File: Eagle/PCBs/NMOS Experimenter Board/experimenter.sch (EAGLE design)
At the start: 1211 parts, among them Q10 2N7002, Q11 2N7002, Q12 2N7002, Q13 2N7002, Q14 2N7002, Q15 2N7002, Q16 2N7002, Q17 2N7002, Q18 2N7002, Q19 2N7002, Q2 2N7002, Q20 2N7002, Q21 2N7002, Q22 2N7002, Q23 2N7002, Q24 2N7002, Q25 2N7002, Q26 2N7002, Q27 2N7002, Q28 2N7002, Q29 2N7002, Q3 2N7002, Q30 2N7002, Q31 2N7002, Q32 2N7002, Q33 2N7002, Q34 2N7002, Q35 2N7002, Q36 2N7002, Q37 2N7002, Q38 2N7002, Q39 2N7002, Q4 2N7002, Q40 2N7002, Q41 2N7002, Q42 2N7002, Q43 2N7002, Q44 2N7002, Q45 2N7002, Q46 2N7002, Q47 2N7002, Q48 2N7002, Q49 2N7002, Q5 2N7002, Q50 2N7002, Q51 2N7002, Q52 2N7002, Q53 2N7002, Q54 2N7002, Q55 2N7002, Q56 2N7002, Q57 2N7002, Q58 2N7002, Q59 2N7002, Q6 2N7002, Q60 2N7002, Q61 2N7002, Q62 2N7002, Q63 2N7002, Q64 2N7002, Q65 2N7002, Q66 2N7002, Q67 2N7002, Q68 2N7002, Q69 2N7002, Q7 2N7002, Q70 2N7002, Q71 2N7002, Q72 2N7002, Q73 2N7002, Q8 2N7002, Q9 2N7002, U1 74HC14PW, U2 74HC14PW

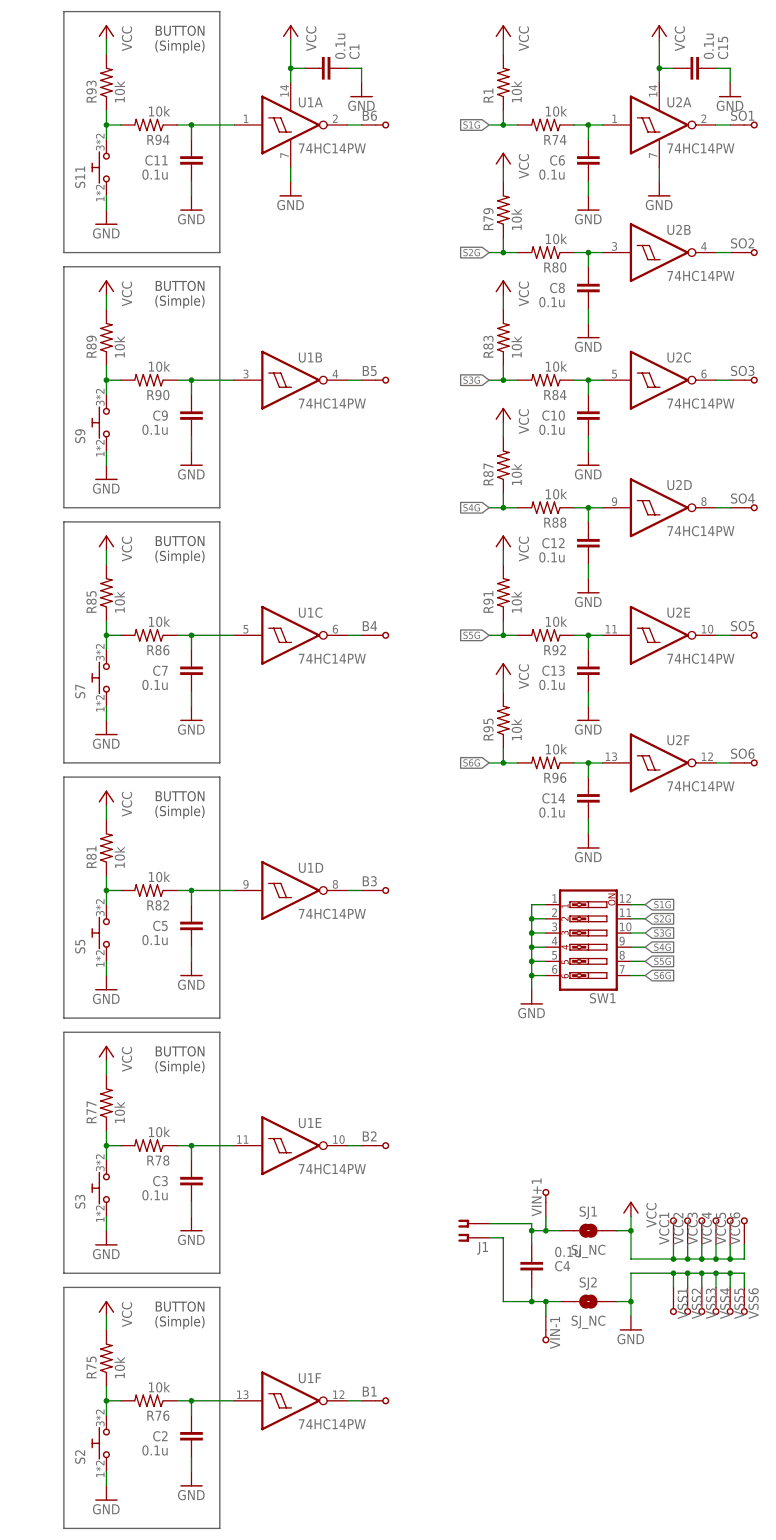
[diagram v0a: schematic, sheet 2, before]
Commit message: Start rework on experimenter
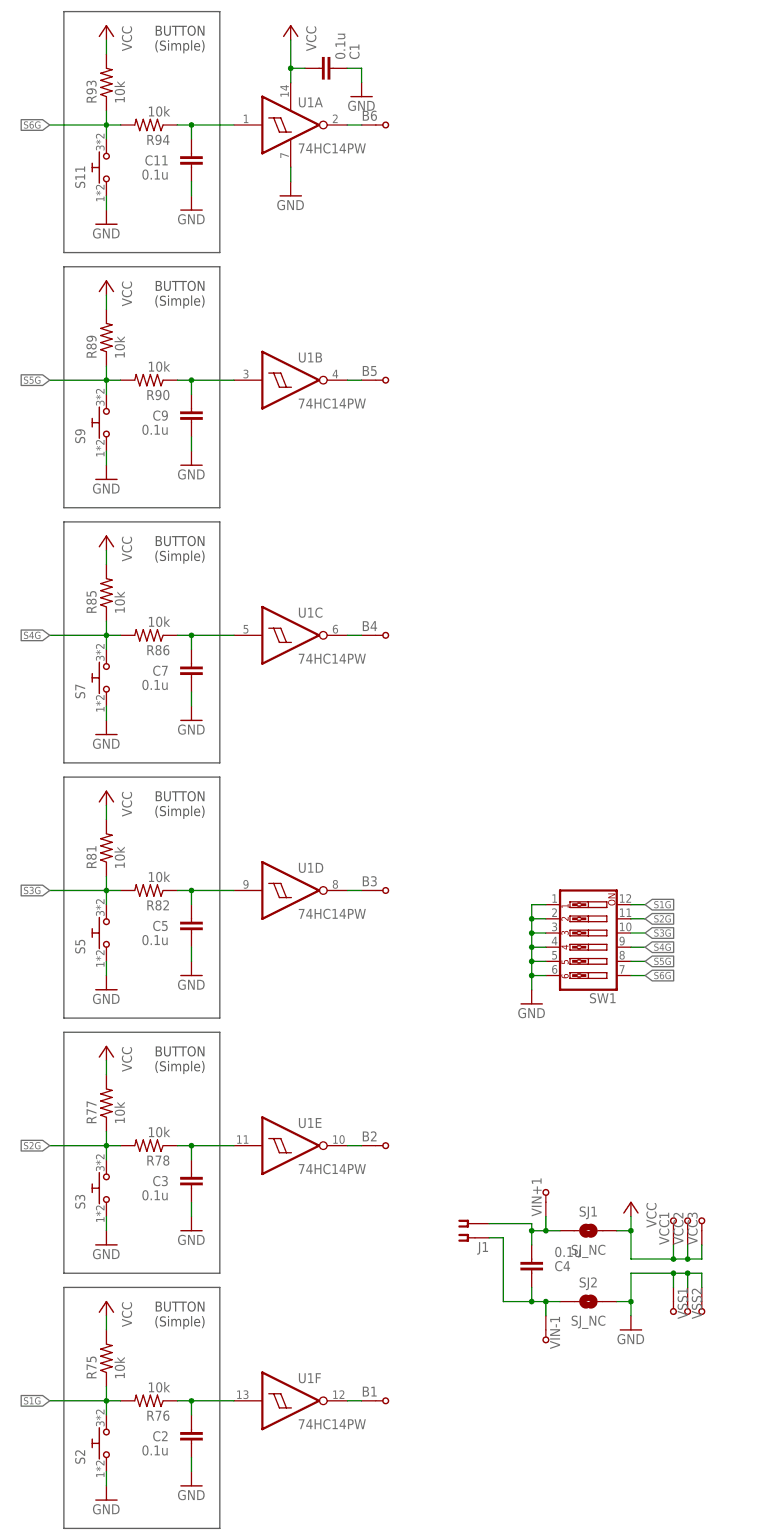
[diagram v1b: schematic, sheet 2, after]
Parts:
- removed C10, C12, C13, C14, C15, C6, C8: 0.1u, ellajameson-core:CAP0603
- removed D10, D11, D12, D13, D14, D15, D16, D17, D18, D19, D2, D20, D21, D22, D23, D24, D25, D26, D27, D28, D29, D3, D30, D31, D32, D33, D34, D35, D36, D37, D38, D39, D4, D40, D41, D42, D43, D44, D45, D46, D47, D48, D49, D5, D50, D51, D52, D53, D54, D55, D56, D57, D58, D59, D6, D60, D61, D62, D63, D64, D65, D66, D67, D68, D69, D7, D70, D71, D72, D73, D8, D9: (no value), ellajameson-core:LED0603
- removed DRAINA10, DRAINA11, DRAINA12, DRAINA13, DRAINA14, DRAINA15, DRAINA16, DRAINA17, DRAINA18, DRAINA19, DRAINA2, DRAINA20, DRAINA21, DRAINA22, DRAINA23, DRAINA24, DRAINA25, DRAINA26, DRAINA27, DRAINA28, DRAINA29, DRAINA3, DRAINA30, DRAINA31, DRAINA32, DRAINA33, DRAINA34, DRAINA35, DRAINA36, DRAINA37, DRAINA38, DRAINA39, DRAINA4, DRAINA40, DRAINA41, DRAINA42, DRAINA43, DRAINA44, DRAINA45, DRAINA46, DRAINA47, DRAINA48, DRAINA49, DRAINA5, DRAINA50, DRAINA51, DRAINA52, DRAINA53, DRAINA54, DRAINA55, DRAINA56, DRAINA57, DRAINA58, DRAINA59, DRAINA6, DRAINA60, DRAINA61, DRAINA62, DRAINA63, DRAINA64, DRAINA65, DRAINA66, DRAINA67, DRAINA68, DRAINA69, DRAINA7, DRAINA70, DRAINA71, DRAINA72, DRAINA73, DRAINA8, DRAINA9, DRAINB10, DRAINB11, DRAINB12, DRAINB13, DRAINB14, DRAINB15, DRAINB16, DRAINB17, DRAINB18, DRAINB19, DRAINB2, DRAINB20, DRAINB21, DRAINB22, DRAINB23, DRAINB24, DRAINB25, DRAINB26, DRAINB27, DRAINB28, DRAINB29, DRAINB3, DRAINB30, DRAINB31, DRAINB32, DRAINB33, DRAINB34, DRAINB35, DRAINB36, DRAINB37, DRAINB38, DRAINB39, DRAINB4, DRAINB40, DRAINB41, DRAINB42, DRAINB43, DRAINB44, DRAINB45, DRAINB46, DRAINB47, DRAINB48, DRAINB49, DRAINB5, DRAINB50, DRAINB51, DRAINB52, DRAINB53, DRAINB54, DRAINB55, DRAINB56, DRAINB57, DRAINB58, DRAINB59, DRAINB6, DRAINB60, DRAINB61, DRAINB62, DRAINB63, DRAINB64, DRAINB65, DRAINB66, DRAINB67, DRAINB68, DRAINB69, DRAINB7, DRAINB70, DRAINB71, DRAINB72, DRAINB73, DRAINB8, DRAINB9, DRAINC10, DRAINC11, DRAINC12, DRAINC13, DRAINC14, DRAINC15, DRAINC16, DRAINC17, DRAINC18, DRAINC19, DRAINC2, DRAINC20, DRAINC21, DRAINC22, DRAINC23, DRAINC24, DRAINC25, DRAINC26, DRAINC27, DRAINC28, DRAINC29, DRAINC3, DRAINC30, DRAINC31, DRAINC32, DRAINC33, DRAINC34, DRAINC35, DRAINC36, DRAINC37, DRAINC38, DRAINC39, DRAINC4, DRAINC40, DRAINC41, DRAINC42, DRAINC43, DRAINC44, DRAINC45, DRAINC46, DRAINC47, DRAINC48, DRAINC49, DRAINC5, DRAINC50, DRAINC51, DRAINC52, DRAINC53, DRAINC54, DRAINC55, DRAINC56, DRAINC57, DRAINC58, DRAINC59, DRAINC6, DRAINC60, DRAINC61, DRAINC62, DRAINC63, DRAINC64, DRAINC65, DRAINC66, DRAINC67, DRAINC68, DRAINC69, DRAINC7, DRAINC70, DRAINC71, DRAINC72, DRAINC73, DRAINC8, DRAINC9, DRAIND10, DRAIND11, DRAIND12, DRAIND13, DRAIND14, DRAIND15, DRAIND16, DRAIND17, DRAIND18, DRAIND19, DRAIND2, DRAIND20, DRAIND21, DRAIND22, DRAIND23, DRAIND24, DRAIND25, DRAIND26, DRAIND27, DRAIND28, DRAIND29, DRAIND3, DRAIND30, DRAIND31, DRAIND32, DRAIND33, DRAIND34, DRAIND35, DRAIND36, DRAIND37, DRAIND38, DRAIND39, DRAIND4, DRAIND40, DRAIND41, DRAIND42, DRAIND43, DRAIND44, DRAIND45, DRAIND46, DRAIND47, DRAIND48, DRAIND49, DRAIND5, DRAIND50, DRAIND51, DRAIND52, DRAIND53, DRAIND54, DRAIND55, DRAIND56, DRAIND57, DRAIND58, DRAIND59, DRAIND6, DRAIND60, DRAIND61, DRAIND62, DRAIND63, DRAIND64, DRAIND65, DRAIND66, DRAIND67, DRAIND68, DRAIND69, DRAIND7, DRAIND70, DRAIND71, DRAIND72, DRAIND73, DRAIND8, DRAIND9, GATE10, GATE11, GATE12, GATE13, GATE14, GATE15, GATE16, GATE17, GATE18, GATE19, GATE2, GATE20, GATE21, GATE22, GATE23, GATE24, GATE25, GATE26, GATE27, GATE28, GATE29, GATE3, GATE30, GATE31, GATE32, GATE33, GATE34, GATE35, GATE36, GATE37, GATE38, GATE39, GATE4, GATE40, GATE41, GATE42, GATE43, GATE44, GATE45, GATE46, GATE47, GATE48, GATE49, GATE5, GATE50, GATE51, GATE52, GATE53, GATE54, GATE55, GATE56, GATE57, GATE58, GATE59, GATE6, GATE60, GATE61, GATE62, GATE63, GATE64, GATE65, GATE66, GATE67, GATE68, GATE69, GATE7, GATE70, GATE71, GATE72, GATE73, GATE8, GATE9, SO1, SO2, SO3, SO4, SO5, SO6, SOURCEA10, SOURCEA11, SOURCEA12, SOURCEA13, SOURCEA14, SOURCEA15, SOURCEA16, SOURCEA17, SOURCEA18, SOURCEA19, SOURCEA2, SOURCEA20, SOURCEA21, SOURCEA22, SOURCEA23, SOURCEA24, SOURCEA25, SOURCEA26, SOURCEA27, SOURCEA28, SOURCEA29, SOURCEA3, SOURCEA30, SOURCEA31, SOURCEA32, SOURCEA33, SOURCEA34, SOURCEA35, SOURCEA36, SOURCEA37, SOURCEA38, SOURCEA39, SOURCEA4, SOURCEA40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: TPWIRE, ellajameson-core:TPWIRE
- removed JD10, JD11, JD12, JD13, JD14, JD17, JD18, JD19, JD2, JD20, JD21, JD22, JD23, JD24, JD25, JD26, JD27, JD28, JD29, JD3, JD30, JD31, JD32, JD33, JD34, JD35, JD36, JD37, JD38, JD39, JD4, JD40, JD41, JD42, JD43, JD44, JD45, JD46, JD47, JD48, JD49, JD5, JD50, JD51, JD52, JD53, JD54, JD55, JD56, JD57, JD58, JD59, JD6, JD60, JD61, JD62, JD63, JD64, JD65, JD66, JD68, JD7, JD70, JD72, JD8, JD9, JN10, JN11, JN12, JN13, JN14, JN15, JN16, JN17, JN18, JN19, JN2, JN20, JN21, JN22, JN23, JN24, JN25, JN26, JN27, JN28, JN29, JN3, JN30, JN31, JN32, JN33, JN34, JN35, JN36, JN37, JN38, JN39, JN4, JN40, JN41, JN42, JN43, JN44, JN45, JN46, JN47, JN48, JN49, JN5, JN50, JN51, JN52, JN53, JN54, JN55, JN56, JN57, JN58, JN59, JN6, JN60, JN61, JN62, JN63, JN64, JN65, JN66, JN67, JN68, JN69, JN7, JN70, JN71, JN72, JN73, JN8, JN9, JP10, JP11, JP12, JP13, JP14, JP15, JP16, JP17, JP18, JP19, JP2, JP20, JP21, JP22, JP23, JP24, JP25, JP26, JP27, JP28, JP29, JP3, JP30, JP31, JP32, JP33, JP34, JP35, JP36, JP37, JP38, JP39, JP4, JP40, JP41, JP42, JP43, JP44, JP45, JP46, JP47, JP48, JP49, JP5, JP50, JP51, JP52, JP53, JP54, JP55, JP56, JP57, JP58, JP59, JP6, JP60, JP61, JP62, JP63, JP64, JP65, JP66, JP67, JP68, JP69, JP7, JP70, JP71, JP72, JP73, JP8, JP9, JS10, JS11, JS12, JS13, JS16, JS17, JS26, JS27, JS28, JS29, JS30, JS31, JS32, JS33, JS34, JS35, JS36, JS37, JS38, JS39, JS4, JS40, JS41, JS42, JS43, JS44, JS45, JS46, JS47, JS48, JS49, JS5, JS50, JS51, JS52, JS53, JS54, JS55, JS56, JS57, JS58, JS59, JS6, JS60, JS61, JS62, JS63, JS64, JS65, JS66, JS67, JS68, JS69, JS7, JS70, JS71, JS72, JS73, JS8, JS9: SJ_NO, ellajameson-core:SJ_NO
- removed Q10, Q11, Q12, Q13, Q14, Q15, Q16, Q17, Q18, Q19, Q2, Q20, Q21, Q22, Q23, Q24, Q25, Q26, Q27, Q28, Q29, Q3, Q30, Q31, Q32, Q33, Q34, Q35, Q36, Q37, Q38, Q39, Q4, Q40, Q41, Q42, Q43, Q44, Q45, Q46, Q47, Q48, Q49, Q5, Q50, Q51, Q52, Q53, Q54, Q55, Q56, Q57, Q58, Q59, Q6, Q60, Q61, Q62, Q63, Q64, Q65, Q66, Q67, Q68, Q69, Q7, Q70, Q71, Q72, Q73, Q8, Q9: 2N7002, ellajameson-core:2N7002
- removed R1, R74, R79, R80, R83, R84, R87, R88, R91, R92, R95, R96: 10k, ellajameson-core:RES0603
- removed R10, R11, R12, R13, R14, R15, R16, R17, R18, R19, R2, R20, R21, R22, R23, R24, R25, R26, R27, R28, R29, R3, R30, R31, R32, R33, R34, R35, R36, R37, R38, R39, R4, R40, R41, R42, R43, R44, R45, R46, R47, R48, R49, R5, R50, R51, R52, R53, R54, R55, R56, R57, R58, R59, R6, R60, R61, R62, R63, R64, R65, R66, R67, R68, R69, R7, R70, R71, R72, R73, R8, R9: (no value), ellajameson-core:RES0603
- removed U2: 74HC14PW, ellajameson-core:74HC14PW
- B1, B2, B3, B4, B5, B6, VCC1, VCC2, VCC3, VIN+1, VIN-1, VSS1, VSS2, VSS3: value TPWIRE -> TPTHT; device ellajameson-core:TPWIRE -> ellajameson-core:TPTHT
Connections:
- removed net N$1: D2.A, JP2.2, R2.1
- removed net N$10: D3.K, DRAINA3.S, DRAINB3.S, DRAINC3.S, DRAIND3.S, JD2.1, JD3.2, JP3.1, JS5.1, Q3.D
- removed net N$100: GATE25.S, Q25.G
- removed net N$101: D26.A, JP26.2, R26.1
- removed net N$102: D26.K, DRAINA26.S, DRAINB26.S, DRAINC26.S, DRAIND26.S, JD26.2, JP26.1, JS34.1, Q26.D
- removed net N$103: JN26.2, JS26.2, Q26.S, SOURCEA26.S, SOURCEB26.S, SOURCEC26.S, SOURCED26.S
- removed net N$104: GATE26.S, Q26.G
- removed net N$105: D27.A, JP27.2, R27.1
- removed net N$106: D27.K, DRAINA27.S, DRAINB27.S, DRAINC27.S, DRAIND27.S, JD26.1, JD27.2, JP27.1, JS35.1, Q27.D
- removed net N$107: JN27.2, JS27.2, Q27.S, SOURCEA27.S, SOURCEB27.S, SOURCEC27.S, SOURCED27.S
- removed net N$108: GATE27.S, Q27.G
- removed net N$109: D28.A, JP28.2, R28.1
- removed net N$11: JN3.2, Q3.S, SOURCEA3.S, SOURCEB3.S, SOURCEC3.S, SOURCED3.S
- removed net N$110: D28.K, DRAINA28.S, DRAINB28.S, DRAINC28.S, DRAIND28.S, JD27.1, JD28.2, JP28.1, JS36.1, Q28.D
- removed net N$111: JN28.2, JS28.2, Q28.S, SOURCEA28.S, SOURCEB28.S, SOURCEC28.S, SOURCED28.S
- removed net N$112: GATE28.S, Q28.G
- removed net N$113: D29.A, JP29.2, R29.1
- removed net N$114: D29.K, DRAINA29.S, DRAINB29.S, DRAINC29.S, DRAIND29.S, JD28.1, JD29.2, JP29.1, JS37.1, Q29.D
- removed net N$115: JN29.2, JS29.2, Q29.S, SOURCEA29.S, SOURCEB29.S, SOURCEC29.S, SOURCED29.S
- removed net N$116: GATE29.S, Q29.G
- removed net N$117: D30.A, JP30.2, R30.1
- removed net N$118: D30.K, DRAINA30.S, DRAINB30.S, DRAINC30.S, DRAIND30.S, JD29.1, JD30.2, JP30.1, JS38.1, Q30.D
- removed net N$119: JN30.2, JS30.2, Q30.S, SOURCEA30.S, SOURCEB30.S, SOURCEC30.S, SOURCED30.S
- removed net N$12: GATE3.S, Q3.G
- removed net N$120: GATE30.S, Q30.G
- removed net N$121: D31.A, JP31.2, R31.1
- removed net N$122: D31.K, DRAINA31.S, DRAINB31.S, DRAINC31.S, DRAIND31.S, JD30.1, JD31.2, JP31.1, JS39.1, Q31.D
- removed net N$123: JN31.2, JS31.2, Q31.S, SOURCEA31.S, SOURCEB31.S, SOURCEC31.S, SOURCED31.S
- removed net N$124: GATE31.S, Q31.G
- removed net N$125: D32.A, JP32.2, R32.1
- removed net N$126: D32.K, DRAINA32.S, DRAINB32.S, DRAINC32.S, DRAIND32.S, JD31.1, JD32.2, JP32.1, JS40.1, Q32.D
- removed net N$127: JN32.2, JS32.2, Q32.S, SOURCEA32.S, SOURCEB32.S, SOURCEC32.S, SOURCED32.S
- removed net N$128: GATE32.S, Q32.G
- removed net N$129: D33.A, JP33.2, R33.1
- removed net N$13: D4.A, JP4.2, R4.1
- removed net N$130: D33.K, DRAINA33.S, DRAINB33.S, DRAINC33.S, DRAIND33.S, JD32.1, JD33.2, JP33.1, JS41.1, Q33.D
- removed net N$131: JN33.2, JS33.2, Q33.S, SOURCEA33.S, SOURCEB33.S, SOURCEC33.S, SOURCED33.S
- removed net N$132: GATE33.S, Q33.G
- removed net N$133: D34.A, JP34.2, R34.1
- removed net N$134: D34.K, DRAINA34.S, DRAINB34.S, DRAINC34.S, DRAIND34.S, JD34.2, JP34.1, JS42.1, Q34.D
- removed net N$135: JN34.2, JS34.2, Q34.S, SOURCEA34.S, SOURCEB34.S, SOURCEC34.S, SOURCED34.S
- removed net N$136: GATE34.S, Q34.G
- removed net N$137: D35.A, JP35.2, R35.1
- removed net N$138: D35.K, DRAINA35.S, DRAINB35.S, DRAINC35.S, DRAIND35.S, JD34.1, JD35.2, JP35.1, JS43.1, Q35.D
- removed net N$139: JN35.2, JS35.2, Q35.S, SOURCEA35.S, SOURCEB35.S, SOURCEC35.S, SOURCED35.S
- removed net N$14: D4.K, DRAINA4.S, DRAINB4.S, DRAINC4.S, DRAIND4.S, JD33.1, JD4.2, JP4.1, JS6.1, Q4.D
- removed net N$140: GATE35.S, Q35.G
- removed net N$141: D36.A, JP36.2, R36.1
- removed net N$142: D36.K, DRAINA36.S, DRAINB36.S, DRAINC36.S, DRAIND36.S, JD35.1, JD36.2, JP36.1, JS44.1, Q36.D
- removed net N$143: JN36.2, JS36.2, Q36.S, SOURCEA36.S, SOURCEB36.S, SOURCEC36.S, SOURCED36.S
- removed net N$144: GATE36.S, Q36.G
- removed net N$145: D37.A, JP37.2, R37.1
- removed net N$146: D37.K, DRAINA37.S, DRAINB37.S, DRAINC37.S, DRAIND37.S, JD36.1, JD37.2, JP37.1, JS45.1, Q37.D
- removed net N$147: JN37.2, JS37.2, Q37.S, SOURCEA37.S, SOURCEB37.S, SOURCEC37.S, SOURCED37.S
- removed net N$148: GATE37.S, Q37.G
- removed net N$149: D38.A, JP38.2, R38.1
- removed net N$15: JN4.2, JS4.2, Q4.S, SOURCEA4.S, SOURCEB4.S, SOURCEC4.S, SOURCED4.S
- removed net N$150: D38.K, DRAINA38.S, DRAINB38.S, DRAINC38.S, DRAIND38.S, JD37.1, JD38.2, JP38.1, JS46.1, Q38.D
- removed net N$151: JN38.2, JS38.2, Q38.S, SOURCEA38.S, SOURCEB38.S, SOURCEC38.S, SOURCED38.S
- removed net N$152: GATE38.S, Q38.G
- removed net N$153: D39.A, JP39.2, R39.1
- removed net N$154: D39.K, DRAINA39.S, DRAINB39.S, DRAINC39.S, DRAIND39.S, JD38.1, JD39.2, JP39.1, JS47.1, Q39.D
- removed net N$155: JN39.2, JS39.2, Q39.S, SOURCEA39.S, SOURCEB39.S, SOURCEC39.S, SOURCED39.S
- removed net N$156: GATE39.S, Q39.G
- removed net N$157: D40.A, JP40.2, R40.1
- removed net N$158: D40.K, DRAINA40.S, DRAINB40.S, DRAINC40.S, DRAIND40.S, JD39.1, JD40.2, JP40.1, JS48.1, Q40.D
- removed net N$159: JN40.2, JS40.2, Q40.S, SOURCEA40.S, SOURCEB40.S, SOURCEC40.S, SOURCED40.S
- removed net N$16: GATE4.S, Q4.G
- removed net N$160: GATE40.S, Q40.G
- removed net N$161: D41.A, JP41.2, R41.1
- removed net N$162: D41.K, DRAINA41.S, DRAINB41.S, DRAINC41.S, DRAIND41.S, JD40.1, JD41.2, JP41.1, JS49.1, Q41.D
- removed net N$163: JN41.2, JS41.2, Q41.S, SOURCEA41.S, SOURCEB41.S, SOURCEC41.S, SOURCED41.S
- removed net N$164: GATE41.S, Q41.G
- removed net N$165: D42.A, JP42.2, R42.1
- removed net N$166: D42.K, DRAINA42.S, DRAINB42.S, DRAINC42.S, DRAIND42.S, JD42.2, JP42.1, JS50.1, Q42.D
- removed net N$167: JN42.2, JS42.2, Q42.S, SOURCEA42.S, SOURCEB42.S, SOURCEC42.S, SOURCED42.S
- removed net N$168: GATE42.S, Q42.G
- removed net N$169: D43.A, JP43.2, R43.1
- removed net N$17: D5.A, JP5.2, R5.1
- removed net N$170: D43.K, DRAINA43.S, DRAINB43.S, DRAINC43.S, DRAIND43.S, JD42.1, JD43.2, JP43.1, JS51.1, Q43.D
- removed net N$171: JN43.2, JS43.2, Q43.S, SOURCEA43.S, SOURCEB43.S, SOURCEC43.S, SOURCED43.S
- removed net N$172: GATE43.S, Q43.G
- removed net N$173: D44.A, JP44.2, R44.1
- removed net N$174: D44.K, DRAINA44.S, DRAINB44.S, DRAINC44.S, DRAIND44.S, JD43.1, JD44.2, JP44.1, JS52.1, Q44.D
- removed net N$175: JN44.2, JS44.2, Q44.S, SOURCEA44.S, SOURCEB44.S, SOURCEC44.S, SOURCED44.S
- removed net N$176: GATE44.S, Q44.G
- removed net N$177: D45.A, JP45.2, R45.1
- removed net N$178: D45.K, DRAINA45.S, DRAINB45.S, DRAINC45.S, DRAIND45.S, JD44.1, JD45.2, JP45.1, JS53.1, Q45.D
- removed net N$179: JN45.2, JS45.2, Q45.S, SOURCEA45.S, SOURCEB45.S, SOURCEC45.S, SOURCED45.S
- removed net N$18: D5.K, DRAINA5.S, DRAINB5.S, DRAINC5.S, DRAIND5.S, JD4.1, JD5.2, JP5.1, JS7.1, Q5.D
- removed net N$180: GATE45.S, Q45.G
- removed net N$181: D46.A, JP46.2, R46.1
- removed net N$182: D46.K, DRAINA46.S, DRAINB46.S, DRAINC46.S, DRAIND46.S, JD45.1, JD46.2, JP46.1, JS54.1, Q46.D
- removed net N$183: JN46.2, JS46.2, Q46.S, SOURCEA46.S, SOURCEB46.S, SOURCEC46.S, SOURCED46.S
- removed net N$184: GATE46.S, Q46.G
- removed net N$185: D47.A, JP47.2, R47.1
- removed net N$186: D47.K, DRAINA47.S, DRAINB47.S, DRAINC47.S, DRAIND47.S, JD46.1, JD47.2, JP47.1, JS55.1, Q47.D
- removed net N$187: JN47.2, JS47.2, Q47.S, SOURCEA47.S, SOURCEB47.S, SOURCEC47.S, SOURCED47.S
- removed net N$188: GATE47.S, Q47.G
- removed net N$189: D48.A, JP48.2, R48.1
- removed net N$19: JN5.2, JS5.2, Q5.S, SOURCEA5.S, SOURCEB5.S, SOURCEC5.S, SOURCED5.S
- removed net N$190: D48.K, DRAINA48.S, DRAINB48.S, DRAINC48.S, DRAIND48.S, JD47.1, JD48.2, JP48.1, JS56.1, Q48.D
- removed net N$191: JN48.2, JS48.2, Q48.S, SOURCEA48.S, SOURCEB48.S, SOURCEC48.S, SOURCED48.S
- removed net N$192: GATE48.S, Q48.G
- removed net N$193: D49.A, JP49.2, R49.1
- removed net N$194: D49.K, DRAINA49.S, DRAINB49.S, DRAINC49.S, DRAIND49.S, JD48.1, JD49.2, JP49.1, JS57.1, Q49.D
- removed net N$195: JN49.2, JS49.2, Q49.S, SOURCEA49.S, SOURCEB49.S, SOURCEC49.S, SOURCED49.S
- removed net N$196: GATE49.S, Q49.G
- removed net N$197: D50.A, JP50.2, R50.1
- removed net N$198: D50.K, DRAINA50.S, DRAINB50.S, DRAINC50.S, DRAIND50.S, JD50.2, JP50.1, JS58.1, Q50.D
- removed net N$199: JN50.2, JS50.2, Q50.S, SOURCEA50.S, SOURCEB50.S, SOURCEC50.S, SOURCED50.S
- removed net N$2: D2.K, DRAINA2.S, DRAINB2.S, DRAINC2.S, DRAIND2.S, JD2.2, JD25.1, JP2.1, JS4.1, Q2.D
- removed net N$20: GATE5.S, Q5.G
- removed net N$200: GATE50.S, Q50.G
- removed net N$201: D51.A, JP51.2, R51.1
- removed net N$202: D51.K, DRAINA51.S, DRAINB51.S, DRAINC51.S, DRAIND51.S, JD50.1, JD51.2, JP51.1, JS59.1, Q51.D
- removed net N$203: JN51.2, JS51.2, Q51.S, SOURCEA51.S, SOURCEB51.S, SOURCEC51.S, SOURCED51.S
- removed net N$204: GATE51.S, Q51.G
- removed net N$205: D52.A, JP52.2, R52.1
- removed net N$206: D52.K, DRAINA52.S, DRAINB52.S, DRAINC52.S, DRAIND52.S, JD51.1, JD52.2, JP52.1, JS60.1, Q52.D
- removed net N$207: JN52.2, JS52.2, Q52.S, SOURCEA52.S, SOURCEB52.S, SOURCEC52.S, SOURCED52.S
- removed net N$208: GATE52.S, Q52.G
- removed net N$209: D53.A, JP53.2, R53.1
- removed net N$21: D6.A, JP6.2, R6.1
- removed net N$210: D53.K, DRAINA53.S, DRAINB53.S, DRAINC53.S, DRAIND53.S, JD52.1, JD53.2, JP53.1, JS61.1, Q53.D
- removed net N$211: JN53.2, JS53.2, Q53.S, SOURCEA53.S, SOURCEB53.S, SOURCEC53.S, SOURCED53.S
- removed net N$212: GATE53.S, Q53.G
- removed net N$213: D54.A, JP54.2, R54.1
- removed net N$214: D54.K, DRAINA54.S, DRAINB54.S, DRAINC54.S, DRAIND54.S, JD53.1, JD54.2, JP54.1, JS62.1, Q54.D
- removed net N$215: JN54.2, JS54.2, Q54.S, SOURCEA54.S, SOURCEB54.S, SOURCEC54.S, SOURCED54.S
- removed net N$216: GATE54.S, Q54.G
- removed net N$217: D55.A, JP55.2, R55.1
- removed net N$218: D55.K, DRAINA55.S, DRAINB55.S, DRAINC55.S, DRAIND55.S, JD54.1, JD55.2, JP55.1, JS63.1, Q55.D
- removed net N$219: JN55.2, JS55.2, Q55.S, SOURCEA55.S, SOURCEB55.S, SOURCEC55.S, SOURCED55.S
- removed net N$22: D6.K, DRAINA6.S, DRAINB6.S, DRAINC6.S, DRAIND6.S, JD41.1, JD6.2, JP6.1, JS8.1, Q6.D
- removed net N$220: GATE55.S, Q55.G
- removed net N$221: D56.A, JP56.2, R56.1
- removed net N$222: D56.K, DRAINA56.S, DRAINB56.S, DRAINC56.S, DRAIND56.S, JD55.1, JD56.2, JP56.1, JS64.1, Q56.D
- removed net N$223: JN56.2, JS56.2, Q56.S, SOURCEA56.S, SOURCEB56.S, SOURCEC56.S, SOURCED56.S
- removed net N$224: GATE56.S, Q56.G
- removed net N$225: D57.A, JP57.2, R57.1
- removed net N$226: D57.K, DRAINA57.S, DRAINB57.S, DRAINC57.S, DRAIND57.S, JD56.1, JD57.2, JP57.1, JS65.1, Q57.D
- removed net N$227: JN57.2, JS57.2, Q57.S, SOURCEA57.S, SOURCEB57.S, SOURCEC57.S, SOURCED57.S
- removed net N$228: GATE57.S, Q57.G
- removed net N$229: D58.A, JP58.2, R58.1
- removed net N$23: JN6.2, JS6.2, Q6.S, SOURCEA6.S, SOURCEB6.S, SOURCEC6.S, SOURCED6.S
- removed net N$230: D58.K, DRAINA58.S, DRAINB58.S, DRAINC58.S, DRAIND58.S, JD58.2, JP58.1, Q58.D
- removed net N$231: JN58.2, JS58.2, Q58.S, SOURCEA58.S, SOURCEB58.S, SOURCEC58.S, SOURCED58.S
- removed net N$232: GATE58.S, Q58.G
- removed net N$233: D59.A, JP59.2, R59.1
- removed net N$234: D59.K, DRAINA59.S, DRAINB59.S, DRAINC59.S, DRAIND59.S, JD58.1, JD59.2, JP59.1, Q59.D
- removed net N$235: JN59.2, JS59.2, Q59.S, SOURCEA59.S, SOURCEB59.S, SOURCEC59.S, SOURCED59.S
- removed net N$236: GATE59.S, Q59.G
- removed net N$237: D60.A, JP60.2, R60.1
- removed net N$238: D60.K, DRAINA60.S, DRAINB60.S, DRAINC60.S, DRAIND60.S, JD59.1, JD60.2, JP60.1, Q60.D
- removed net N$239: JN60.2, JS60.2, Q60.S, SOURCEA60.S, SOURCEB60.S, SOURCEC60.S, SOURCED60.S
- removed net N$24: GATE6.S, Q6.G
- removed net N$240: GATE60.S, Q60.G
- removed net N$241: D61.A, JP61.2, R61.1
- removed net N$242: D61.K, DRAINA61.S, DRAINB61.S, DRAINC61.S, DRAIND61.S, JD60.1, JD61.2, JP61.1, Q61.D
- removed net N$243: JN61.2, JS61.2, Q61.S, SOURCEA61.S, SOURCEB61.S, SOURCEC61.S, SOURCED61.S
- removed net N$244: GATE61.S, Q61.G
- removed net N$245: D62.A, JP62.2, R62.1
- removed net N$246: D62.K, DRAINA62.S, DRAINB62.S, DRAINC62.S, DRAIND62.S, JD61.1, JD62.2, JP62.1, Q62.D
- removed net N$247: JN62.2, JS62.2, Q62.S, SOURCEA62.S, SOURCEB62.S, SOURCEC62.S, SOURCED62.S
- removed net N$248: GATE62.S, Q62.G
- removed net N$249: D63.A, JP63.2, R63.1
- removed net N$25: D7.A, JP7.2, R7.1
- removed net N$250: D63.K, DRAINA63.S, DRAINB63.S, DRAINC63.S, DRAIND63.S, JD62.1, JD63.2, JP63.1, Q63.D
- removed net N$251: JN63.2, JS63.2, Q63.S, SOURCEA63.S, SOURCEB63.S, SOURCEC63.S, SOURCED63.S
- removed net N$252: GATE63.S, Q63.G
- removed net N$253: D64.A, JP64.2, R64.1
- removed net N$254: D64.K, DRAINA64.S, DRAINB64.S, DRAINC64.S, DRAIND64.S, JD63.1, JD64.2, JP64.1, Q64.D
- removed net N$255: JN64.2, JS64.2, Q64.S, SOURCEA64.S, SOURCEB64.S, SOURCEC64.S, SOURCED64.S
- removed net N$256: GATE64.S, Q64.G
- removed net N$257: D65.A, JP65.2, R65.1
- removed net N$258: D65.K, DRAINA65.S, DRAINB65.S, DRAINC65.S, DRAIND65.S, JD64.1, JD65.2, JP65.1, Q65.D
- removed net N$259: JN65.2, JS65.2, Q65.S, SOURCEA65.S, SOURCEB65.S, SOURCEC65.S, SOURCED65.S
- removed net N$26: D7.K, DRAINA7.S, DRAINB7.S, DRAINC7.S, DRAIND7.S, JD6.1, JD7.2, JP7.1, JS9.1, Q7.D
- removed net N$260: GATE65.S, Q65.G
- removed net N$261: D66.A, JP66.2, R66.1
- removed net N$262: D66.K, DRAINA66.S, DRAINB66.S, DRAINC66.S, DRAIND66.S, JD66.2, JD7.1, JP66.1, JS68.1, Q66.D
- removed net N$263: JN66.2, JS66.2, Q66.S, SOURCEA66.S, SOURCEB66.S, SOURCEC66.S, SOURCED66.S
- removed net N$264: GATE66.S, Q66.G
- removed net N$265: D67.A, JP67.2, R67.1
- removed net N$266: D67.K, DRAINA67.S, DRAINB67.S, DRAINC67.S, DRAIND67.S, JD66.1, JP67.1, JS69.1, Q67.D
- removed net N$267: JN67.2, JS67.2, Q67.S, SOURCEA67.S, SOURCEB67.S, SOURCEC67.S, SOURCED67.S
- removed net N$268: GATE67.S, Q67.G
- removed net N$269: D68.A, JP68.2, R68.1
- removed net N$27: JN7.2, JS7.2, Q7.S, SOURCEA7.S, SOURCEB7.S, SOURCEC7.S, SOURCED7.S
- removed net N$270: D68.K, DRAINA68.S, DRAINB68.S, DRAINC68.S, DRAIND68.S, JD68.2, JD9.1, JP68.1, JS70.1, Q68.D
- removed net N$271: JN68.2, JS68.2, Q68.S, SOURCEA68.S, SOURCEB68.S, SOURCEC68.S, SOURCED68.S
- removed net N$272: GATE68.S, Q68.G
- removed net N$273: D69.A, JP69.2, R69.1
- removed net N$274: D69.K, DRAINA69.S, DRAINB69.S, DRAINC69.S, DRAIND69.S, JD68.1, JP69.1, JS71.1, Q69.D
- removed net N$275: JN69.2, JS69.2, Q69.S, SOURCEA69.S, SOURCEB69.S, SOURCEC69.S, SOURCED69.S
- removed net N$276: GATE69.S, Q69.G
- removed net N$277: D70.A, JP70.2, R70.1
- removed net N$278: D70.K, DRAINA70.S, DRAINB70.S, DRAINC70.S, DRAIND70.S, JD11.1, JD70.2, JP70.1, JS72.1, Q70.D
- removed net N$279: JN70.2, JS70.2, Q70.S, SOURCEA70.S, SOURCEB70.S, SOURCEC70.S, SOURCED70.S
- removed net N$28: GATE7.S, Q7.G
- removed net N$280: GATE70.S, Q70.G
- removed net N$281: D71.A, JP71.2, R71.1
- removed net N$282: D71.K, DRAINA71.S, DRAINB71.S, DRAINC71.S, DRAIND71.S, JD70.1, JP71.1, JS73.1, Q71.D
- removed net N$283: JN71.2, JS71.2, Q71.S, SOURCEA71.S, SOURCEB71.S, SOURCEC71.S, SOURCED71.S
- removed net N$284: GATE71.S, Q71.G
- removed net N$285: D72.A, JP72.2, R72.1
- removed net N$286: D72.K, DRAINA72.S, DRAINB72.S, DRAINC72.S, DRAIND72.S, JD13.1, JD72.2, JP72.1, Q72.D
- removed net N$287: JN72.2, JS72.2, Q72.S, SOURCEA72.S, SOURCEB72.S, SOURCEC72.S, SOURCED72.S
- removed net N$288: GATE72.S, Q72.G
- removed net N$289: D73.A, JP73.2, R73.1
- removed net N$29: D8.A, JP8.2, R8.1
- removed net N$290: D73.K, DRAINA73.S, DRAINB73.S, DRAINC73.S, DRAIND73.S, JD72.1, JP73.1, Q73.D
- removed net N$291: JN73.2, JS73.2, Q73.S, SOURCEA73.S, SOURCEB73.S, SOURCEC73.S, SOURCED73.S
- removed net N$292: GATE73.S, Q73.G
- removed net N$293: R77.1, R78.2, S3.S
- removed net N$297: R81.1, R82.2, S5.S
- removed net N$3: JN2.2, Q2.S, SOURCEA2.S, SOURCEB2.S, SOURCEC2.S, SOURCED2.S
- removed net N$30: D8.K, DRAINA8.S, DRAINB8.S, DRAINC8.S, DRAIND8.S, JD49.1, JD8.2, JP8.1, JS10.1, Q8.D
- removed net N$301: R85.1, R86.2, S7.S
- removed net N$305: R89.1, R90.2, S9.S
- removed net N$307: SO6.S, U2F.O
- removed net N$308: SO5.S, U2E.O
- removed net N$309: R93.1, R94.2, S11.S
- removed net N$31: JN8.2, JS8.2, Q8.S, SOURCEA8.S, SOURCEB8.S, SOURCEC8.S, SOURCED8.S
- removed net N$311: SO4.S, U2D.O
- removed net N$312: C8.1, R80.1, U2B.I
- removed net N$313: SO3.S, U2C.O
- removed net N$314: C10.1, R84.1, U2C.I
- removed net N$315: SO2.S, U2B.O
- removed net N$316: C12.1, R88.1, U2D.I
- removed net N$317: SO1.S, U2A.O
- removed net N$318: C13.1, R92.1, U2E.I
- removed net N$32: GATE8.S, Q8.G
- removed net N$320: C14.1, R96.1, U2F.I
- removed net N$33: D9.A, JP9.2, R9.1
- removed net N$34: D9.K, DRAINA9.S, DRAINB9.S, DRAINC9.S, DRAIND9.S, JD8.1, JD9.2, JP9.1, JS11.1, Q9.D
- removed net N$35: JN9.2, JS9.2, Q9.S, SOURCEA9.S, SOURCEB9.S, SOURCEC9.S, SOURCED9.S
- removed net N$36: GATE9.S, Q9.G
- removed net N$37: D10.A, JP10.2, R10.1
- removed net N$38: D10.K, DRAINA10.S, DRAINB10.S, DRAINC10.S, DRAIND10.S, JD10.2, JD57.1, JP10.1, JS12.1, Q10.D
- removed net N$39: JN10.2, JS10.2, Q10.S, SOURCEA10.S, SOURCEB10.S, SOURCEC10.S, SOURCED10.S
- removed net N$4: GATE2.S, Q2.G
- removed net N$40: GATE10.S, Q10.G
- removed net N$41: D11.A, JP11.2, R11.1
- removed net N$42: D11.K, DRAINA11.S, DRAINB11.S, DRAINC11.S, DRAIND11.S, JD10.1, JD11.2, JP11.1, JS13.1, Q11.D
- removed net N$43: JN11.2, JS11.2, Q11.S, SOURCEA11.S, SOURCEB11.S, SOURCEC11.S, SOURCED11.S
- removed net N$44: GATE11.S, Q11.G
- removed net N$45: D12.A, JP12.2, R12.1
- removed net N$46: D12.K, DRAINA12.S, DRAINB12.S, DRAINC12.S, DRAIND12.S, JD12.2, JD65.1, JP12.1, Q12.D
- removed net N$47: JN12.2, JS12.2, Q12.S, SOURCEA12.S, SOURCEB12.S, SOURCEC12.S, SOURCED12.S
- removed net N$48: GATE12.S, Q12.G
- removed net N$49: D13.A, JP13.2, R13.1
- removed net N$50: D13.K, DRAINA13.S, DRAINB13.S, DRAINC13.S, DRAIND13.S, JD12.1, JD13.2, JP13.1, Q13.D
- removed net N$51: JN13.2, JS13.2, Q13.S, SOURCEA13.S, SOURCEB13.S, SOURCEC13.S, SOURCED13.S
- removed net N$52: GATE13.S, Q13.G
- removed net N$53: D14.A, JP14.2, R14.1
- removed net N$54: D14.K, DRAINA14.S, DRAINB14.S, DRAINC14.S, DRAIND14.S, JD14.2, JD3.1, JP14.1, JS17.1, Q14.D
- removed net N$55: JN14.2, Q14.S, SOURCEA14.S, SOURCEB14.S, SOURCEC14.S, SOURCED14.S
- removed net N$56: GATE14.S, Q14.G
- removed net N$57: D15.A, JP15.2, R15.1
- removed net N$58: D15.K, DRAINA15.S, DRAINB15.S, DRAINC15.S, DRAIND15.S, JD14.1, JP15.1, JS16.1, Q15.D
- removed net N$59: JN15.2, Q15.S, SOURCEA15.S, SOURCEB15.S, SOURCEC15.S, SOURCED15.S
- removed net N$60: GATE15.S, Q15.G
- removed net N$61: D16.A, JP16.2, R16.1
- removed net N$62: D16.K, DRAINA16.S, DRAINB16.S, DRAINC16.S, DRAIND16.S, JD17.1, JP16.1, JS67.1, Q16.D
- removed net N$63: JN16.2, JS16.2, Q16.S, SOURCEA16.S, SOURCEB16.S, SOURCEC16.S, SOURCED16.S
- removed net N$64: GATE16.S, Q16.G
- removed net N$65: D17.A, JP17.2, R17.1
- removed net N$66: D17.K, DRAINA17.S, DRAINB17.S, DRAINC17.S, DRAIND17.S, JD17.2, JD5.1, JP17.1, JS66.1, Q17.D
- removed net N$67: JN17.2, JS17.2, Q17.S, SOURCEA17.S, SOURCEB17.S, SOURCEC17.S, SOURCED17.S
- removed net N$68: GATE17.S, Q17.G
- removed net N$69: D18.A, JP18.2, R18.1
- removed net N$7: R75.1, R76.2, S2.S
- removed net N$70: D18.K, DRAINA18.S, DRAINB18.S, DRAINC18.S, DRAIND18.S, JD18.2, JP18.1, JS26.1, Q18.D
- removed net N$71: JN18.2, Q18.S, SOURCEA18.S, SOURCEB18.S, SOURCEC18.S, SOURCED18.S
- removed net N$72: GATE18.S, Q18.G
- removed net N$73: D19.A, JP19.2, R19.1
- removed net N$74: D19.K, DRAINA19.S, DRAINB19.S, DRAINC19.S, DRAIND19.S, JD18.1, JD19.2, JP19.1, JS27.1, Q19.D
- removed net N$75: JN19.2, Q19.S, SOURCEA19.S, SOURCEB19.S, SOURCEC19.S, SOURCED19.S
- removed net N$76: GATE19.S, Q19.G
- removed net N$77: D20.A, JP20.2, R20.1
- removed net N$78: D20.K, DRAINA20.S, DRAINB20.S, DRAINC20.S, DRAIND20.S, JD19.1, JD20.2, JP20.1, JS28.1, Q20.D
- removed net N$79: JN20.2, Q20.S, SOURCEA20.S, SOURCEB20.S, SOURCEC20.S, SOURCED20.S
- removed net N$80: GATE20.S, Q20.G
- removed net N$81: D21.A, JP21.2, R21.1
- removed net N$82: D21.K, DRAINA21.S, DRAINB21.S, DRAINC21.S, DRAIND21.S, JD20.1, JD21.2, JP21.1, JS29.1, Q21.D
- removed net N$83: JN21.2, Q21.S, SOURCEA21.S, SOURCEB21.S, SOURCEC21.S, SOURCED21.S
- removed net N$84: GATE21.S, Q21.G
- removed net N$85: D22.A, JP22.2, R22.1
- removed net N$86: D22.K, DRAINA22.S, DRAINB22.S, DRAINC22.S, DRAIND22.S, JD21.1, JD22.2, JP22.1, JS30.1, Q22.D
- removed net N$87: JN22.2, Q22.S, SOURCEA22.S, SOURCEB22.S, SOURCEC22.S, SOURCED22.S
- removed net N$88: GATE22.S, Q22.G
- removed net N$89: D23.A, JP23.2, R23.1
- removed net N$9: D3.A, JP3.2, R3.1
- removed net N$90: D23.K, DRAINA23.S, DRAINB23.S, DRAINC23.S, DRAIND23.S, JD22.1, JD23.2, JP23.1, JS31.1, Q23.D
- removed net N$91: JN23.2, Q23.S, SOURCEA23.S, SOURCEB23.S, SOURCEC23.S, SOURCED23.S
- removed net N$92: GATE23.S, Q23.G
- removed net N$93: D24.A, JP24.2, R24.1
- removed net N$94: D24.K, DRAINA24.S, DRAINB24.S, DRAINC24.S, DRAIND24.S, JD23.1, JD24.2, JP24.1, JS32.1, Q24.D
- removed net N$95: JN24.2, Q24.S, SOURCEA24.S, SOURCEB24.S, SOURCEC24.S, SOURCED24.S
- removed net N$96: GATE24.S, Q24.G
- removed net N$97: D25.A, JP25.2, R25.1
- removed net N$98: D25.K, DRAINA25.S, DRAINB25.S, DRAINC25.S, DRAIND25.S, JD24.1, JD25.2, JP25.1, JS33.1, Q25.D
- removed net N$99: JN25.2, Q25.S, SOURCEA25.S, SOURCEB25.S, SOURCEC25.S, SOURCED25.S
- removed net S1F: C6.1, R74.1, U2A.I
- net GND: no longer C10.2, C12.2, C13.2, C14.2, C15.2, C6.2, C8.2, JN10.1, JN11.1, JN12.1, JN13.1, JN14.1, JN15.1, JN16.1, JN17.1, JN18.1, JN19.1, JN2.1, JN20.1, JN21.1, JN22.1, JN23.1, JN24.1, JN25.1, JN26.1, JN27.1, JN28.1, JN29.1, JN3.1, JN30.1, JN31.1, JN32.1, JN33.1, JN34.1, JN35.1, JN36.1, JN37.1, JN38.1, JN39.1, JN4.1, JN40.1, JN41.1, JN42.1, JN43.1, JN44.1, JN45.1, JN46.1, JN47.1, JN48.1, JN49.1, JN5.1, JN50.1, JN51.1, JN52.1, JN53.1, JN54.1, JN55.1, JN56.1, JN57.1, JN58.1, JN59.1, JN6.1, JN60.1, JN61.1, JN62.1, JN63.1, JN64.1, JN65.1, JN66.1, JN67.1, JN68.1, JN69.1, JN7.1, JN70.1, JN71.1, JN72.1, JN73.1, JN8.1, JN9.1, U2G$1.V-, VSS4.S, VSS5.S, VSS6.S
- net S1G: now also R75.1, R76.2, S2.S; no longer R1.1, R74.2
- net S2G: now also R77.1, R78.2, S3.S; no longer R79.1, R80.2
- net S3G: now also R81.1, R82.2, S5.S; no longer R83.1, R84.2
- net S4G: now also R85.1, R86.2, S7.S; no longer R87.1, R88.2
- net S5G: now also R89.1, R90.2, S9.S; no longer R91.1, R92.2
- net S6G: now also R93.1, R94.2, S11.S; no longer R95.1, R96.2
- net VCC: no longer C15.1, R1.2, R10.2, R11.2, R12.2, R13.2, R14.2, R15.2, R16.2, R17.2, R18.2, R19.2, R2.2, R20.2, R21.2, R22.2, R23.2, R24.2, R25.2, R26.2, R27.2, R28.2, R29.2, R3.2, R30.2, R31.2, R32.2, R33.2, R34.2, R35.2, R36.2, R37.2, R38.2, R39.2, R4.2, R40.2, R41.2, R42.2, R43.2, R44.2, R45.2, R46.2, R47.2, R48.2, R49.2, R5.2, R50.2, R51.2, R52.2, R53.2, R54.2, R55.2, R56.2, R57.2, R58.2, R59.2, R6.2, R60.2, R61.2, R62.2, R63.2, R64.2, R65.2, R66.2, R67.2, R68.2, R69.2, R7.2, R70.2, R71.2, R72.2, R73.2, R79.2, R8.2, R83.2, R87.2, R9.2, R91.2, R95.2, U2G$1.V+, VCC4.S, VCC5.S, VCC6.S
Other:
- note removed: "NMOS Logic Transistor Cell"
